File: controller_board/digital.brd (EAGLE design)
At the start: 148 x 129.2 mm, 34 parts

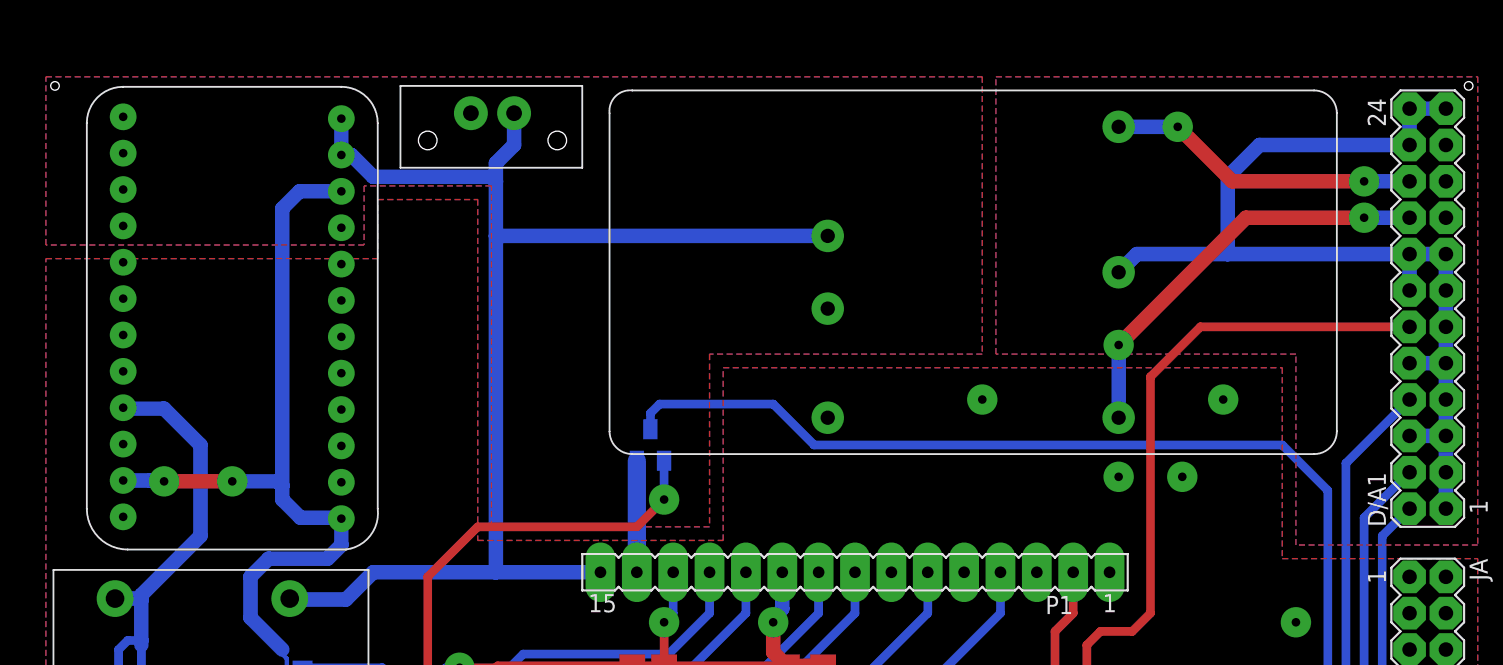
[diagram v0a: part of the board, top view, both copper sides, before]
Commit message: Changes to Electronics Design
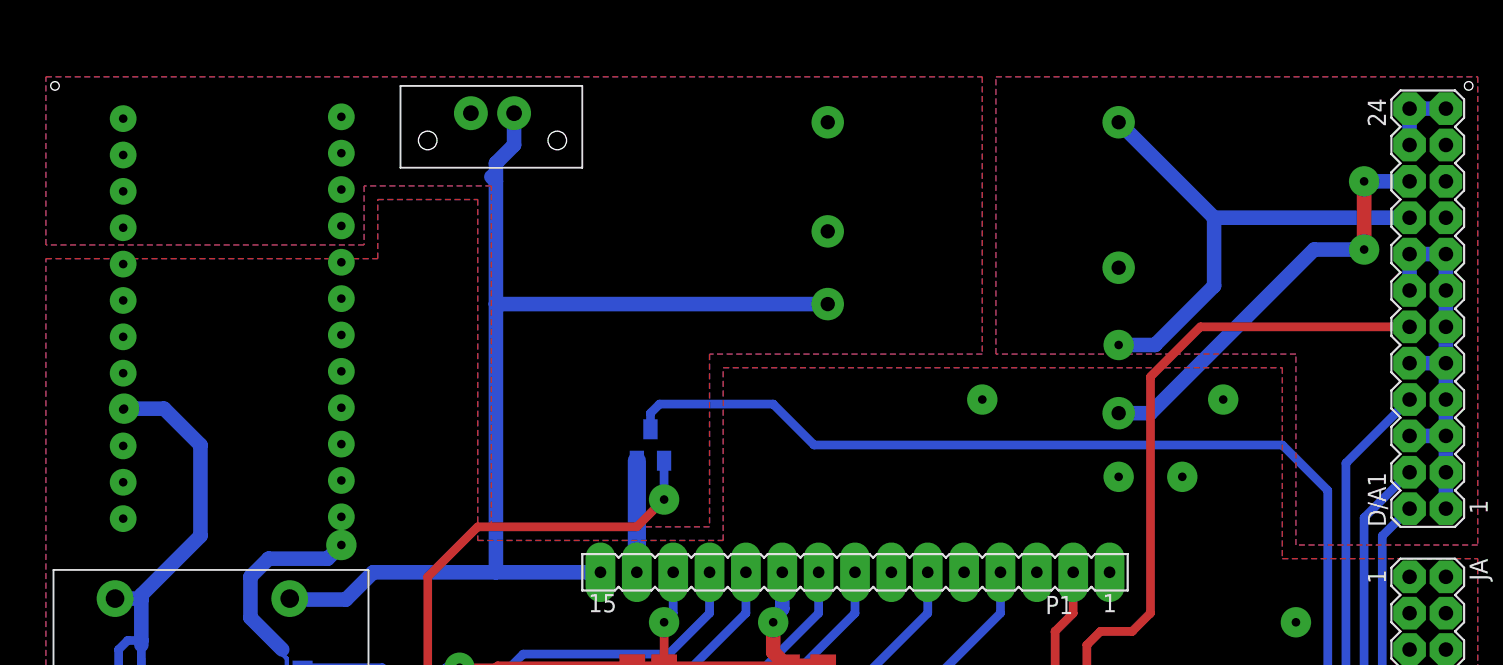
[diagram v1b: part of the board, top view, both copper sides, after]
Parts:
- moved U$28 25.1 mm to (39.4, 54.0), flipped to the bottom, turned to 180 degrees
- moved U$46 11.4 mm to (13.0, 68.9), flipped to the bottom, turned to 180 degrees
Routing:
- net GNDD: track 200.3 -> 157.6 mm, vias 23 -> 22
- net GNDA: track 72.2 -> 32.4 mm
- net VBATT: track 92.4 -> 78.7 mm
- net +15V: track 21.9 -> 29.8 mm
- net -15V: track 29.1 -> 36.2 mm, vias 2 -> 1
- net +5V: track 185.1 -> 185.0 mm, vias 7 -> 8
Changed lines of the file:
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@@
 <attribute name="OC_NEWARK" value="unknown" x="96.52" y="16.51" size="1.778" layer="27" rot="R90" display="off"/>
 </element>
-<element name="U$28" library="custom_parts" package="TEN20-4823" value="TEN20-4823WIN" x="39.37" y="79.0575"/>
+<element name="U$28" library="custom_parts" package="TEN20-4823" value="TEN20-4823WIN" x="39.37" y="53.975" rot="MR180"/>
 <element name="U$36" library="custom_parts" package="SOT23-5L" value="SN74LVC1G17" x="85.09" y="13.335" rot="MR0"/>
-<element name="U$46" library="custom_parts" package="DIP24" value="TVN5-4811WI" x="13.0175" y="57.4675"/>
+<element name="U$46" library="custom_parts" package="DIP24" value="TVN5-4811WI" x="13.0175" y="68.8975" rot="MR180"/>
 <element name="U$49" library="custom_parts" package="JS1-5V-F" value="JS1-5V-F" x="11.43" y="37.465"/>
 <element name="U$55" library="custom_parts" package="MICROFIT-3.0" value="MICROFIT" x="29.21" y="76.835"/>
@@
 <wire x1="87.9475" y1="13.335" x2="85.4075" y2="13.335" width="0.6096" layer="16"/>
 <wire x1="85.4075" y1="13.335" x2="85.09" y2="13.6525" width="0.6096" layer="16"/>
-<wire x1="20.6375" y1="72.009" x2="17.7165" y2="72.009" width="1.016" layer="16"/>
-<wire x1="17.7165" y1="72.009" x2="16.51" y2="70.8025" width="1.016" layer="16"/>
-<wire x1="16.51" y1="70.8025" x2="16.51" y2="51.435" width="1.016" layer="16"/>
 <wire x1="15.5575" y1="46.355" x2="14.2875" y2="45.085" width="1.016" layer="16"/>
 <wire x1="14.2875" y1="45.085" x2="14.2875" y2="42.2275" width="1.016" layer="16"/>
@@
 <via x="66.675" y="13.0175" extent="1-16" drill="0.6"/>
 <contactref element="U$5" pad="2"/>
-<wire x1="5.3975" y1="51.816" x2="7.239" y2="51.816" width="1.016" layer="16"/>
-<wire x1="7.239" y1="51.816" x2="8.255" y2="51.7525" width="1.016" layer="16"/>
-<via x="8.255" y="51.7525" extent="1-16" drill="0.6"/>
-<wire x1="8.255" y1="51.7525" x2="13.0175" y2="51.7525" width="1.016" layer="1"/>
-<via x="13.0175" y="51.7525" extent="1-16" drill="0.6"/>
-<wire x1="13.0175" y1="51.7525" x2="16.1925" y2="51.7525" width="1.016" layer="16"/>
-<wire x1="16.1925" y1="51.7525" x2="16.51" y2="51.435" width="1.016" layer="16"/>
-<wire x1="16.51" y1="51.435" x2="16.51" y2="50.4825" width="1.016" layer="16"/>
-<wire x1="16.51" y1="50.4825" x2="17.78" y2="49.2125" width="1.016" layer="16"/>
-<wire x1="17.78" y1="49.2125" x2="20.574" y2="49.2125" width="1.016" layer="16"/>
-<wire x1="20.574" y1="49.2125" x2="20.6375" y2="49.149" width="1.016" layer="16"/>
 <wire x1="15.5575" y1="46.355" x2="19.685" y2="46.355" width="1.016" layer="16"/>
 <wire x1="19.685" y1="46.355" x2="20.6375" y2="47.3075" width="1.016" layer="16"/>
-<wire x1="20.6375" y1="47.3075" x2="20.6375" y2="49.149" width="1.016" layer="16"/>
 <wire x1="22.225" y1="36.83" x2="23.495" y2="35.56" width="0.6096" layer="16"/>
 <wire x1="23.495" y1="35.56" x2="25.7175" y2="35.56" width="0.6096" layer="16"/>
@@
 <via x="48.26" y="30.7975" extent="1-16" drill="0.6"/>
 <via x="54.2925" y="31.115" extent="1-16" drill="0.6"/>
+<via x="20.6375" y="47.3075" extent="1-16" drill="0.6"/>
+<wire x1="5.3975" y1="74.549" x2="20.6375" y2="77.216" width="0" layer="19" extent="1-1"/>
+<wire x1="20.6375" y1="54.356" x2="20.6375" y2="77.216" width="0" layer="19" extent="1-1"/>
 </signal>
 <signal name="ADC_M2">
@@
 <vertex x="87.3125" y="60.6425"/>
 </polygon>
-<wire x1="95.25" y1="67.6275" x2="82.55" y2="67.6275" width="1.016" layer="16"/>
-<wire x1="82.55" y1="67.6275" x2="76.2" y2="67.6275" width="1.016" layer="16"/>
-<wire x1="76.2" y1="67.6275" x2="74.93" y2="66.3575" width="1.016" layer="16"/>
-<wire x1="95.25" y1="75.2475" x2="84.7725" y2="75.2475" width="1.016" layer="16"/>
-<wire x1="84.7725" y1="75.2475" x2="82.55" y2="73.025" width="1.016" layer="16"/>
-<wire x1="82.55" y1="73.025" x2="82.55" y2="67.6275" width="1.016" layer="16"/>
 </signal>
 <signal name="VBATT">
@@
 <contactref element="U$46" pad="P$1"/>
 <contactref element="U$46" pad="P$2"/>
+<wire x1="38.735" y1="45.4025" x2="31.4325" y2="45.4025" width="1.016" layer="16"/>
 <wire x1="31.4325" y1="45.4025" x2="22.86" y2="45.4025" width="1.016" layer="16"/>
 <wire x1="22.86" y1="45.4025" x2="20.955" y2="43.4975" width="1.016" layer="16"/>
 <wire x1="20.955" y1="43.4975" x2="17.0975" y2="43.4975" width="1.016" layer="16"/>
 <wire x1="17.0975" y1="43.4975" x2="17.03" y2="43.565" width="1.016" layer="16"/>
-<wire x1="20.6375" y1="77.089" x2="20.6375" y2="74.549" width="1.016" layer="16"/>
-<wire x1="38.735" y1="45.4025" x2="31.4325" y2="45.4025" width="1.016" layer="16"/>
-<wire x1="31.4325" y1="72.7075" x2="31.4325" y2="68.8975" width="1.016" layer="16"/>
-<wire x1="31.4325" y1="68.8975" x2="31.4325" y2="45.4025" width="1.016" layer="16"/>
-<wire x1="54.61" y1="68.8975" x2="31.4325" y2="68.8975" width="1.016" layer="16"/>
-<wire x1="20.6375" y1="74.549" x2="21.336" y2="74.549" width="1.016" layer="16"/>
-<wire x1="21.336" y1="74.549" x2="22.86" y2="73.025" width="1.016" layer="16"/>
-<wire x1="22.86" y1="73.025" x2="31.115" y2="73.025" width="1.016" layer="16"/>
 <wire x1="31.115" y1="73.025" x2="31.4325" y2="72.7075" width="1.016" layer="16"/>
 <wire x1="31.4325" y1="72.7075" x2="31.4325" y2="73.9775" width="1.016" layer="16"/>
 <wire x1="31.4325" y1="73.9775" x2="32.7025" y2="75.2475" width="1.016" layer="16"/>
 <wire x1="32.7025" y1="75.2475" x2="32.7025" y2="77.47" width="1.016" layer="16"/>
+<wire x1="31.4325" y1="72.7075" x2="31.4325" y2="64.135" width="1.016" layer="16"/>
+<wire x1="31.4325" y1="64.135" x2="31.4325" y2="45.4025" width="1.016" layer="16"/>
+<wire x1="54.61" y1="64.135" x2="31.4325" y2="64.135" width="1.016" layer="16"/>
+<wire x1="20.6375" y1="49.276" x2="20.6375" y2="51.816" width="0" layer="19" extent="1-1"/>
+<wire x1="22.86" y1="45.4025" x2="20.6375" y2="49.276" width="0" layer="19" extent="16-16"/>
 </signal>
 <signal name="GNDP">
@@
 <wire x1="41.275" y1="45.4025" x2="41.2775" y2="45.4025" width="1.016" layer="16"/>
 <wire x1="41.2775" y1="45.4025" x2="41.2775" y2="53.1925" width="1.27" layer="16"/>
+<wire x1="5.3975" y1="49.149" x2="5.3975" y2="51.689" width="0" layer="19" extent="1-1"/>
+<wire x1="29.68625" y1="77.47" x2="5.3975" y2="51.689" width="0" layer="19" extent="1-1"/>
 </signal>
 <signal name="DRIVE_ENABLE">
@@
 <contactref element="U$28" pad="P$5"/>
 <contactref element="D/A1" pad="18"/>
-<wire x1="95.25" y1="70.1675" x2="92.075" y2="70.1675" width="1.016" layer="16"/>
-<via x="92.075" y="70.1675" extent="1-16" drill="0.6"/>
-<wire x1="92.075" y1="70.1675" x2="83.82" y2="70.1675" width="1.016" layer="1"/>
-<wire x1="83.82" y1="70.1675" x2="74.93" y2="61.2775" width="1.016" layer="1"/>
 <via x="74.93" y="61.2775" extent="1-16" drill="0.6"/>
-<wire x1="74.93" y1="61.2775" x2="74.93" y2="56.1975" width="1.016" layer="16"/>
+<wire x1="95.25" y1="70.1675" x2="81.5975" y2="70.1675" width="1.016" layer="16"/>
+<wire x1="81.5975" y1="70.1675" x2="74.93" y2="76.835" width="1.016" layer="16"/>
+<wire x1="74.93" y1="61.2775" x2="77.47" y2="61.2775" width="1.016" layer="16"/>
+<wire x1="77.47" y1="61.2775" x2="81.5975" y2="65.405" width="1.016" layer="16"/>
+<wire x1="81.5975" y1="65.405" x2="81.5975" y2="70.1675" width="1.016" layer="16"/>
 </signal>
 <signal name="N$42">
@@
 <wire x1="14" y1="22.55" x2="15.2325" y2="22.55" width="1.016" layer="1"/>
 <wire x1="15.2325" y1="22.55" x2="15.24" y2="22.5425" width="1.016" layer="1"/>
-<wire x1="5.461" y1="56.8325" x2="5.3975" y2="56.896" width="1.016" layer="16"/>
+<wire x1="5.461" y1="56.8325" x2="5.3975" y2="69.469" width="0" layer="19" extent="1-16"/>
 <wire x1="8.255" y1="56.8325" x2="5.461" y2="56.8325" width="1.016" layer="16"/>
 <wire x1="88.265" y1="16.8275" x2="88.265" y2="18.7325" width="0.6096" layer="1"/>
@@
 <wire x1="18.415" y1="23.1775" x2="17.145" y2="23.1775" width="0.6096" layer="1"/>
 <wire x1="17.145" y1="23.1775" x2="16.8275" y2="22.86" width="0.6096" layer="1"/>
+<via x="5.461" y="56.8325" extent="1-16" drill="0.6"/>
 </signal>
 <signal name="N$5">
@@
 <wire x1="95.25" y1="72.7075" x2="92.075" y2="72.7075" width="1.016" layer="16"/>
 <via x="92.075" y="72.7075" extent="1-16" drill="0.6"/>
-<wire x1="92.075" y1="72.7075" x2="82.8675" y2="72.7075" width="1.016" layer="1"/>
-<wire x1="82.8675" y1="72.7075" x2="79.0575" y2="76.5175" width="1.016" layer="1"/>
-<via x="79.0575" y="76.5175" extent="1-16" drill="0.6"/>
-<wire x1="79.0575" y1="76.5175" x2="74.93" y2="76.5175" width="1.016" layer="16"/>
+<wire x1="88.5825" y1="67.945" x2="77.1525" y2="56.515" width="1.016" layer="16"/>
+<wire x1="77.1525" y1="56.515" x2="74.93" y2="56.515" width="1.016" layer="16"/>
+<wire x1="92.075" y1="72.7075" x2="92.075" y2="67.945" width="1.016" layer="1"/>
+<via x="92.075" y="67.945" extent="1-16" drill="0.6"/>
+<wire x1="92.075" y1="67.945" x2="88.5825" y2="67.945" width="1.016" layer="16"/>
 </signal>
 <signal name="OTP_EN_GATE">
